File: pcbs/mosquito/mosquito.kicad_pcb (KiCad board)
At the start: 2 copper layers, 131.4 x 84.2 mm, 23 parts, among them SW1 SW_PUSH, SW10 SW_PUSH, SW11 SW_PUSH, SW12 SW_PUSH, SW13 SW_PUSH, SW14 SW_PUSH, SW15 SW_PUSH, SW16 SW_PUSH, SW17 SW_PUSH, SW2 SW_PUSH, SW3 SW_PUSH, SW4 SW_PUSH, SW5 SW_PUSH, SW6 SW_PUSH, SW7 SW_PUSH, SW8 SW_PUSH, SW9 SW_PUSH, U1 ProMicro

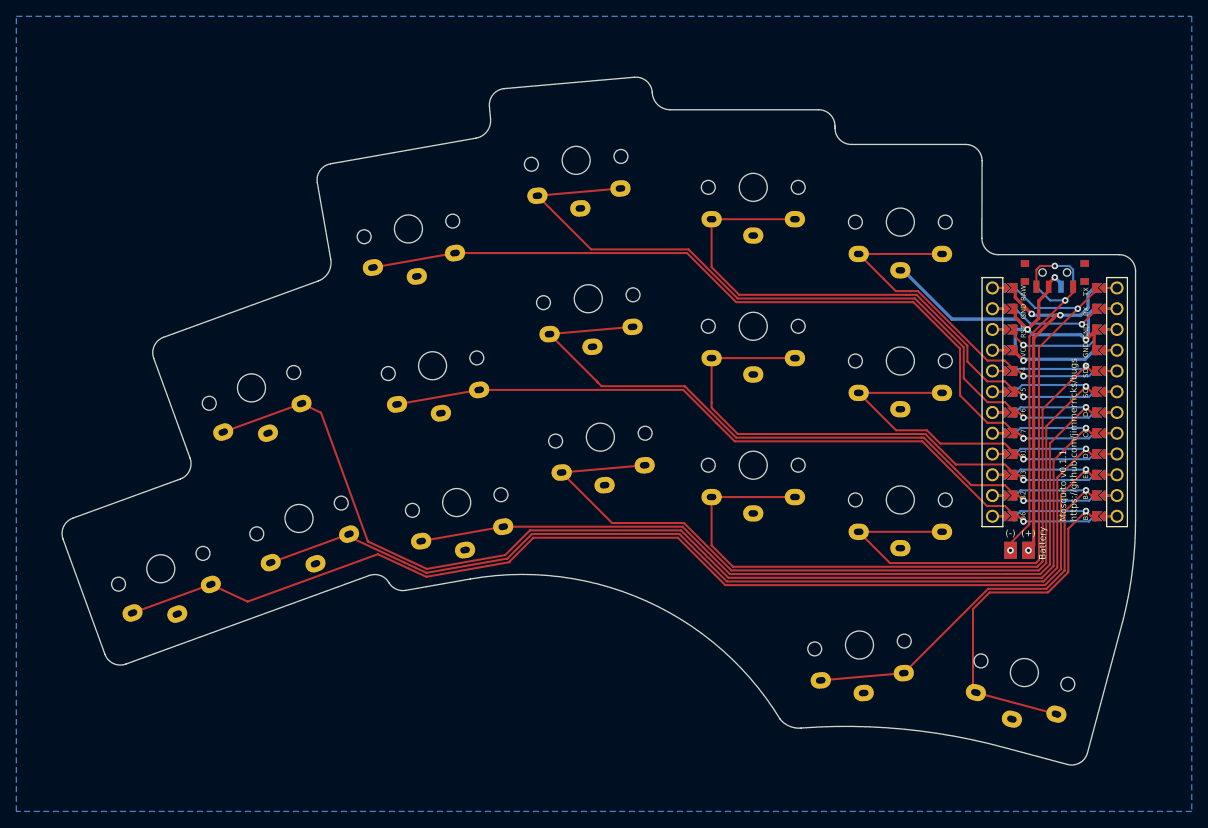
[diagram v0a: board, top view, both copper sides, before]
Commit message: Update gnat & mosquito edge
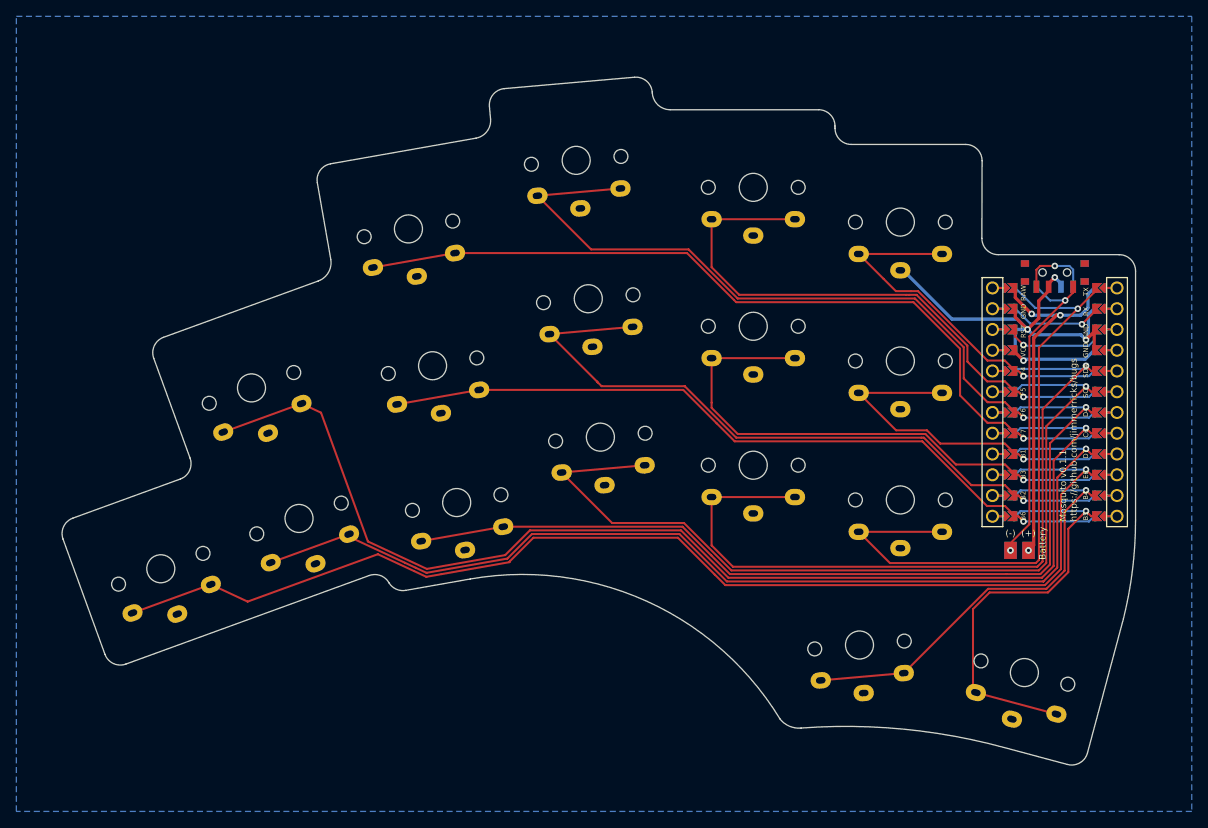
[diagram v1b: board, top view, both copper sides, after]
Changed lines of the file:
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@@
-(kicad_pcb (version 20210925) (generator pcbnew)
+(kicad_pcb (version 20211014) (generator pcbnew)
   (general
     (thickness 1.6)
@@
     )
   )
-  (gr_arc (start 65.286162 100.026216) (end 63.597443 101.107088) (angle -67.37913673) (layer "Edge.Cuts") (width 0.15))
+  (gr_arc (start 65.634348 102.00076) (mid 64.480606 101.862282) (end 63.597443 101.107088) (layer "Edge.Cuts") (width 0.15))
   (gr_line (start 65.634349 102.000758) (end 73.513304 100.611484) (layer "Edge.Cuts") (width 0.15))
   (gr_line (start 35.987812 71.036376) (end 54.923833 64.144229) (layer "Edge.Cuts") (width 0.15))
   (gr_line (start 61.164893 100.183602) (end 31.386239 111.022147) (layer "Edge.Cuts") (width 0.15))
-  (gr_arc (start 77.860625 42.596754) (end 77.686316 40.604356) (angle -90) (layer "Edge.Cuts") (width 0.15))
-  (gr_arc (start 105.013421 93.391973) (end 153.45182 105.470751) (angle -14.00185829) (layer "Edge.Cuts") (width 0.15))
-  (gr_arc (start 61.845985 102.055063) (end 63.597443 101.107088) (angle -81.57382184) (layer "Edge.Cuts") (width 0.15))
+  (gr_arc (start 75.868227 42.771063) (mid 76.328532 41.311171) (end 77.686316 40.604356) (layer "Edge.Cuts") (width 0.15))
+  (gr_arc (start 154.935113 93.392031) (mid 154.562899 99.476758) (end 153.45182 105.470751) (layer "Edge.Cuts") (width 0.15))
+  (gr_arc (start 61.164893 100.1836) (mid 62.552829 100.193174) (end 63.597443 101.107088) (layer "Edge.Cuts") (width 0.15))
   (gr_line (start 23.692335 95.730941) (end 28.822809 109.826805) (layer "Edge.Cuts") (width 0.15))
-  (gr_arc (start 152.935241 62.924752) (end 154.935243 62.924753) (angle -90) (layer "Edge.Cuts") (width 0.15))
+  (gr_arc (start 152.935242 60.92475) (mid 154.349457 61.510538) (end 154.935243 62.924753) (layer "Edge.Cuts") (width 0.15))
   (gr_line (start 118.154857 45.185603) (end 118.155247 45.434747) (layer "Edge.Cuts") (width 0.15))
-  (gr_line (start 138.874253 121.234546) (end 146.601651 123.305096) (layer "Edge.Cuts") (width 0.15))
+  (gr_line (start 138.874246 121.234543) (end 146.601651 123.305096) (layer "Edge.Cuts") (width 0.15))
   (gr_line (start 95.792131 41.027948) (end 95.806599 41.193318) (layer "Edge.Cuts") (width 0.15))
-  (gr_arc (start 56.778257 51.774894) (end 56.430959 49.805279) (angle -90) (layer "Edge.Cuts") (width 0.15))
-  (gr_arc (start 73.834624 44.520255) (end 74.213634 46.669711) (angle -84.99985992) (layer "Edge.Cuts") (width 0.15))
-  (gr_arc (start 37.359472 86.49954) (end 38.043509 88.378931) (angle -90) (layer "Edge.Cuts") (width 0.15))
-  (gr_line (start 138.129369 60.924744) (end 152.935244 60.924756) (layer "Edge.Cuts") (width 0.15))
-  (gr_arc (start 119.477018 192.621122) (end 114.011546 118.848331) (angle 19.43846695) (layer "Edge.Cuts") (width 0.15))
-  (gr_arc (start 36.671844 72.91577) (end 35.987812 71.036376) (angle -90) (layer "Edge.Cuts") (width 0.15))
-  (gr_line (start 120.155254 47.43475) (end 134.155033 47.434967) (layer "Edge.Cuts") (width 0.15))
-  (gr_arc (start 147.119292 121.373246) (end 146.601651 123.305096) (angle -90) (layer "Edge.Cuts") (width 0.15))
-  (gr_line (start 149.051144 121.890881) (end 153.45182 105.470751) (layer "Edge.Cuts") (width 0.15))
-  (gr_arc (start 134.155032 49.43497) (end 136.155032 49.43497) (angle -90) (layer "Edge.Cuts") (width 0.15))
+  (gr_arc (start 54.808642 52.122192) (mid 55.139952 50.627743) (end 56.430959 49.805279) (layer "Edge.Cuts") (width 0.15))
+  (gr_arc (start 76.008934 44.33003) (mid 75.566209 45.848947) (end 74.213634 46.669711) (layer "Edge.Cuts") (width 0.15))
+  (gr_arc (start 39.238863 85.815503) (mid 39.172089 87.344783) (end 38.043509 88.378931) (layer "Edge.Cuts") (width 0.15))
+  (gr_line (start 138.129376 60.924752) (end 152.935242 60.92475) (layer "Edge.Cuts") (width 0.15))
+  (gr_arc (start 114.011546 118.848331) (mid 126.544334 118.98452) (end 138.874246 121.234543) (layer "Edge.Cuts") (width 0.15))
+  (gr_arc (start 34.79245 73.599802) (mid 34.859228 72.070521) (end 35.987812 71.036376) (layer "Edge.Cuts") (width 0.15))
+  (gr_line (start 120.155241 47.434753) (end 134.155032 47.43497) (layer "Edge.Cuts") (width 0.15))
+  (gr_arc (start 149.051142 121.890887) (mid 148.119289 123.105298) (end 146.601651 123.305096) (layer "Edge.Cuts") (width 0.15))
+  (gr_line (start 149.051142 121.890887) (end 153.45182 105.470751) (layer "Edge.Cuts") (width 0.15))
+  (gr_arc (start 134.155032 47.43497) (mid 135.569246 48.020756) (end 136.155032 49.43497) (layer "Edge.Cuts") (width 0.15))
   (gr_line (start 24.887681 93.167516) (end 38.043509 88.378931) (layer "Edge.Cuts") (width 0.15))
-  (gr_arc (start 30.702195 109.142763) (end 28.822809 109.826805) (angle -90) (layer "Edge.Cuts") (width 0.15))
-  (gr_line (start 154.935243 62.924753) (end 154.935116 93.39203) (layer "Edge.Cuts") (width 0.15))
-  (gr_arc (start 120.155247 45.434753) (end 118.155247 45.434747) (angle -90) (layer "Edge.Cuts") (width 0.15))
-  (gr_line (start 97.98091 43.185703) (end 116.154859 43.185599) (layer "Edge.Cuts") (width 0.15))
-  (gr_arc (start 113.752873 115.892621) (end 111.44512 117.765095) (angle -55.94629929) (layer "Edge.Cuts") (width 0.15))
-  (gr_arc (start 97.980901 41.003087) (end 95.806599 41.193318) (angle -85.00013873) (layer "Edge.Cuts") (width 0.15))
-  (gr_line (start 56.455924 61.490581) (end 54.808637 52.122188) (layer "Edge.Cuts") (width 0.15))
-  (gr_arc (start 54.108625 61.904469) (end 54.923833 64.144229) (angle -79.99998711) (layer "Edge.Cuts") (width 0.15))
-  (gr_arc (start 93.79974 41.202258) (end 95.792131 41.027948) (angle -90) (layer "Edge.Cuts") (width 0.15))
-  (gr_line (start 34.792462 73.599808) (end 39.23886 85.815503) (layer "Edge.Cuts") (width 0.15))
-  (gr_arc (start 79.921782 136.95656) (end 111.44512 117.765095) (angle -68.66666424) (layer "Edge.Cuts") (width 0.15))
-  (gr_line (start 75.868239 42.771062) (end 76.008934 44.330029) (layer "Edge.Cuts") (width 0.15))
-  (gr_line (start 77.686316 40.604356) (end 93.625432 39.209869) (layer "Edge.Cuts") (width 0.15))
+  (gr_arc (start 31.386237 111.022149) (mid 29.856959 110.95538) (end 28.822809 109.826805) (layer "Edge.Cuts") (width 0.15))
+  (gr_line (start 154.935243 62.924753) (end 154.935113 93.392031) (layer "Edge.Cuts") (width 0.15))
+  (gr_arc (start 120.155241 47.434753) (mid 118.741029 46.848962) (end 118.155247 45.434747) (layer "Edge.Cuts") (width 0.15))
+  (gr_line (start 97.98091 43.185695) (end 116.154866 43.1856) (layer "Edge.Cuts") (width 0.15))
+  (gr_arc (start 114.011971 118.853153) (mid 112.593039 118.628798) (end 111.44512 117.765095) (layer "Edge.Cuts") (width 0.15))
+  (gr_arc (start 97.98091 43.185695) (mid 96.506357 42.612279) (end 95.806599 41.193318) (layer "Edge.Cuts") (width 0.15))
+  (gr_line (start 56.455917 61.490577) (end 54.808642 52.122192) (layer "Edge.Cuts") (width 0.15))
+  (gr_arc (start 56.455917 61.490577) (mid 56.1728 63.096219) (end 54.923833 64.144229) (layer "Edge.Cuts") (width 0.15))
+  (gr_arc (start 93.62543 39.209867) (mid 95.085317 39.670169) (end 95.792131 41.027948) (layer "Edge.Cuts") (width 0.15))
+  (gr_line (start 34.79245 73.599802) (end 39.23886 85.815503) (layer "Edge.Cuts") (width 0.15))
+  (gr_arc (start 73.513299 100.611485) (mid 95.128707 103.329449) (end 111.44512 117.765095) (layer "Edge.Cuts") (width 0.15))
+  (gr_line (start 75.868227 42.771063) (end 76.008934 44.33003) (layer "Edge.Cuts") (width 0.15))
+  (gr_line (start 77.686316 40.604356) (end 93.62543 39.209867) (layer "Edge.Cuts") (width 0.15))
   (gr_line (start 56.430959 49.805279) (end 74.213634 46.669711) (layer "Edge.Cuts") (width 0.15))
-  (gr_arc (start 116.15486 45.185597) (end 118.154857 45.185603) (angle -90) (layer "Edge.Cuts") (width 0.15))
-  (gr_arc (start 25.571721 95.046904) (end 24.887681 93.167516) (angle -90) (layer "Edge.Cuts") (width 0.15))
+  (gr_arc (start 116.154866 43.1856) (mid 117.569076 43.77139) (end 118.154857 45.185603) (layer "Edge.Cuts") (width 0.15))
+  (gr_arc (start 23.692333 95.730944) (mid 23.759104 94.201665) (end 24.887681 93.167516) (layer "Edge.Cuts") (width 0.15))
   (gr_line (start 136.155032 49.43497) (end 136.129374 58.924756) (layer "Edge.Cuts") (width 0.15))
-  (gr_arc (start 138.129373 58.924753) (end 136.129374 58.924756) (angle -90) (layer "Edge.Cuts") (width 0.15))
+  (gr_arc (start 138.129376 60.924752) (mid 136.715162 60.338968) (end 136.129374 58.924756) (layer "Edge.Cuts") (width 0.15))
   (gr_text "Mosquito v0.1.1\nhttps://github.com/jimmerricks/bugs" (at 146.710002 70.360004 90) (layer "B.SilkS")
     (effects (font (size 0.8 0.8) (thickness 0.1)) (justify left mirror))
